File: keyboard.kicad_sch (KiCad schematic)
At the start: 33 parts, among them IC2 80C51, IC3 74LS145, IC4 74LS145, IC7 74LS366, IC9 74LS241

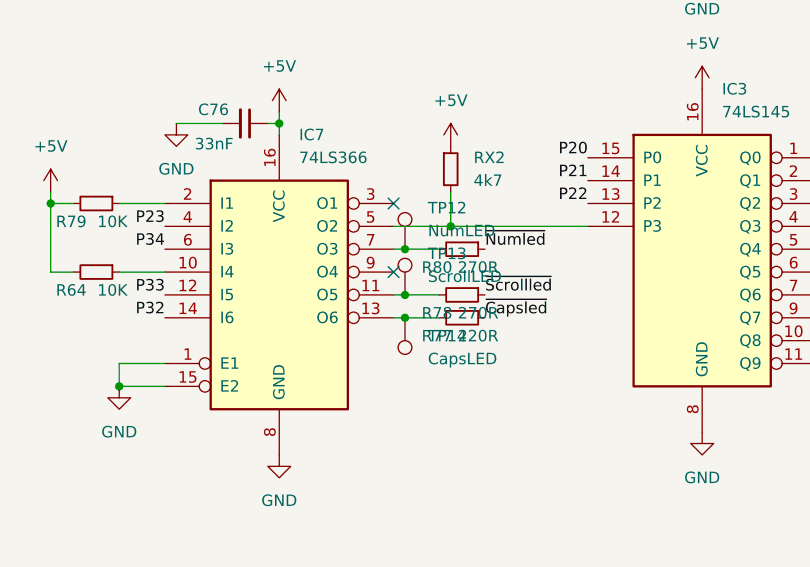
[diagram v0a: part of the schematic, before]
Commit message: prepare for fabrication
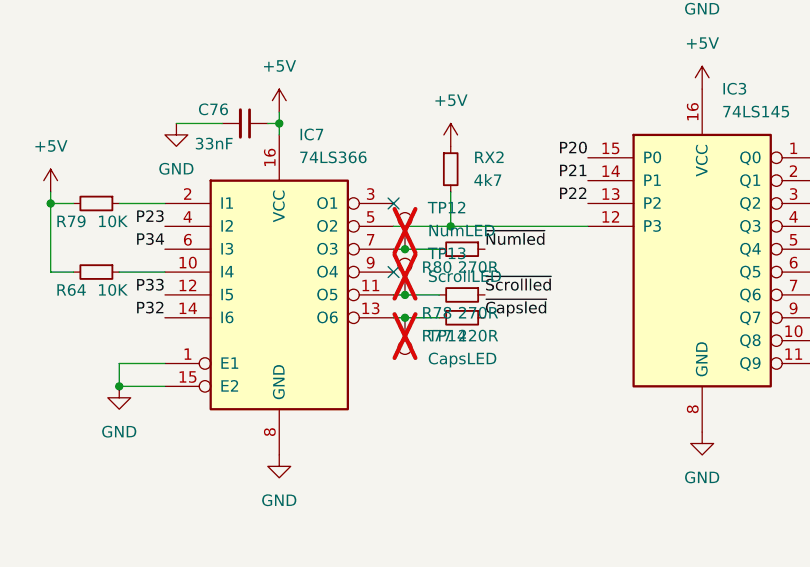
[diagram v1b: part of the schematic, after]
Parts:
- C76, C77, C87: LCSC (none) -> C344201; LCSC Part (none) -> C344201
- IC3, IC4: LCSC (none) -> C60829; LCSC Part (none) -> C60829
- IC9: LCSC (none) -> C2676097; LCSC Part (none) -> C2676097
- R49: LCSC (none) -> C2907326; LCSC Part (none) -> C2907326
- R64, R79: LCSC (none) -> C2907219; LCSC Part (none) -> C2907219
- R71, R72: LCSC (none) -> C17630; LCSC Part (none) -> C17630
- R77: LCSC (none) -> C17557; LCSC Part (none) -> C17557
- R78, R80: LCSC (none) -> C17590; LCSC Part (none) -> C17590
- RP3: LCSC (none) -> C1739866; LCSC Part (none) -> C1739866
- TP12, TP13, TP14: now not fitted
